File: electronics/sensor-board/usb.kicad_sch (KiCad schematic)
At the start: 1 part

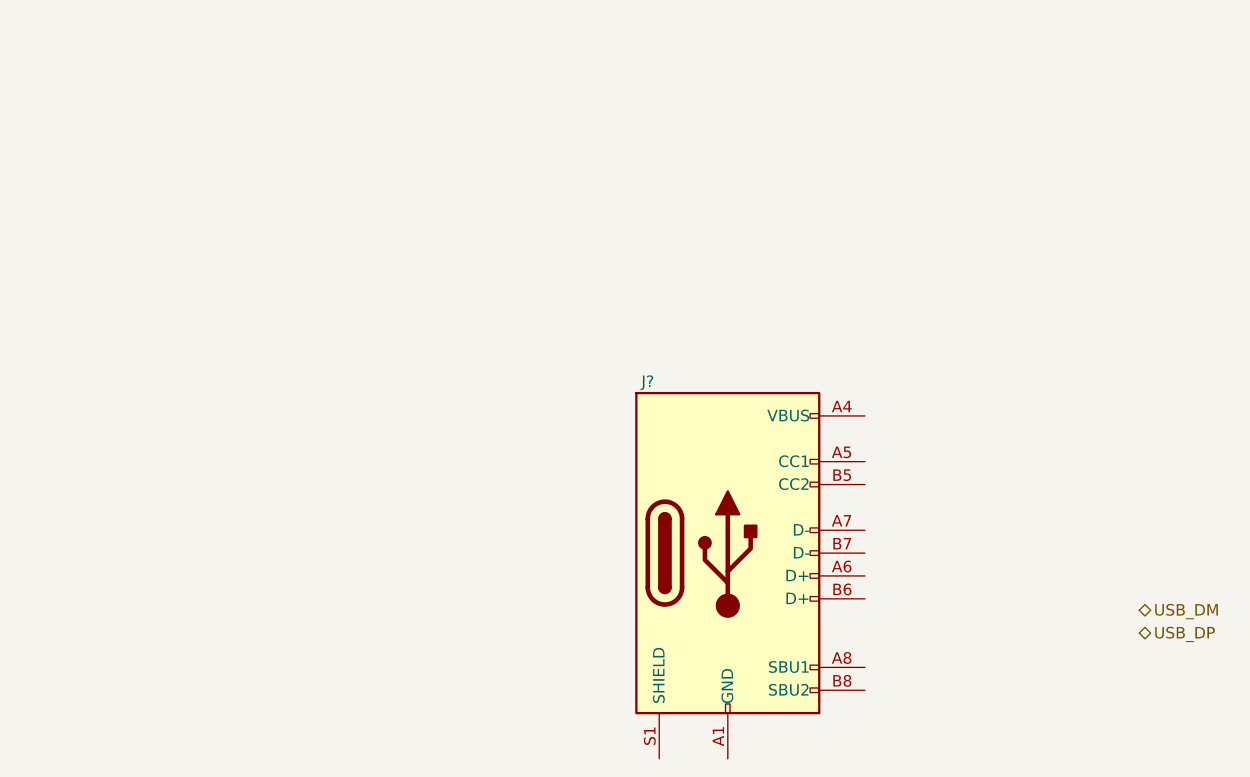
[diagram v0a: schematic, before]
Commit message: Finalize USB
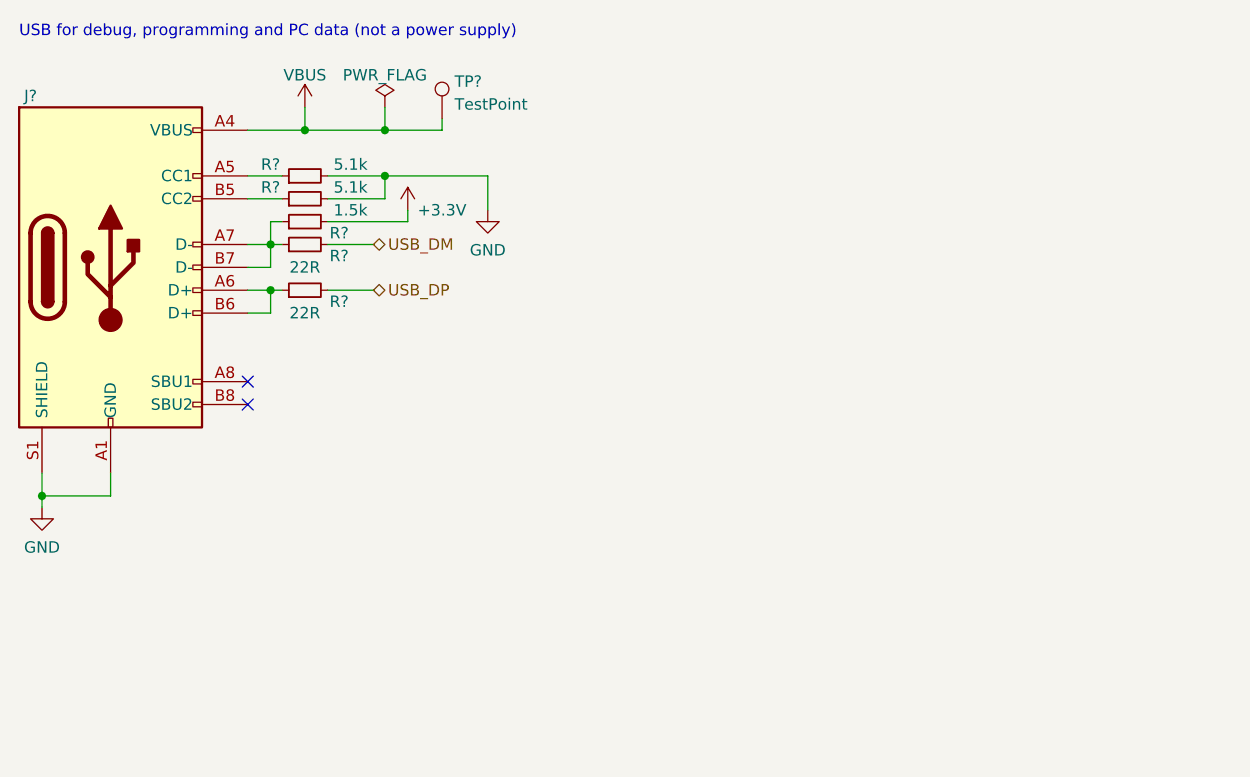
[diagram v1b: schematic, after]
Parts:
- added R?: 1.5k, symbol Device:R_Small
- added R? (x2): 5.1k, symbol Device:R_Small
- added R? (x2): 22R, symbol Device:R_Small
- added TP?: TestPoint, symbol Connector:TestPoint
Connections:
- net USB_DM: now also R?.2
- net USB_DP: now also R?.2
- net GND: now reaches J?.A1 (GND), J?.A12 (GND), J?.B1 (GND), J?.B12 (GND)
- net GND: now also J?.S1 (SHIELD), R?.2, R?.2
- net VBUS: now reaches J?.A4 (VBUS), J?.A9 (VBUS), J?.B4 (VBUS), J?.B9 (VBUS)
- net VBUS: now also TP?.1
- net at J?.A5 (CC1): now also R?.1
- net at J?.A6 (D+): now also J?.B6 (D+), R?.1
- net at J?.A7 (D-): now also J?.B7 (D-), R?.1, R?.1
- net at J?.B5 (CC2): now also R?.1
- new net +3.3V: R?.2
- no-connect marks 0 -> 2
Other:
- note added: "USB for debug, programming and PC data (not a power supply)"
- moved on the sheet: J?
